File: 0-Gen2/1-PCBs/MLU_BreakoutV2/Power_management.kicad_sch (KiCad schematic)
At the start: 11 parts, among them J6 430450228, SW1 09.03201.02, U1 BA033CC0FP-E2

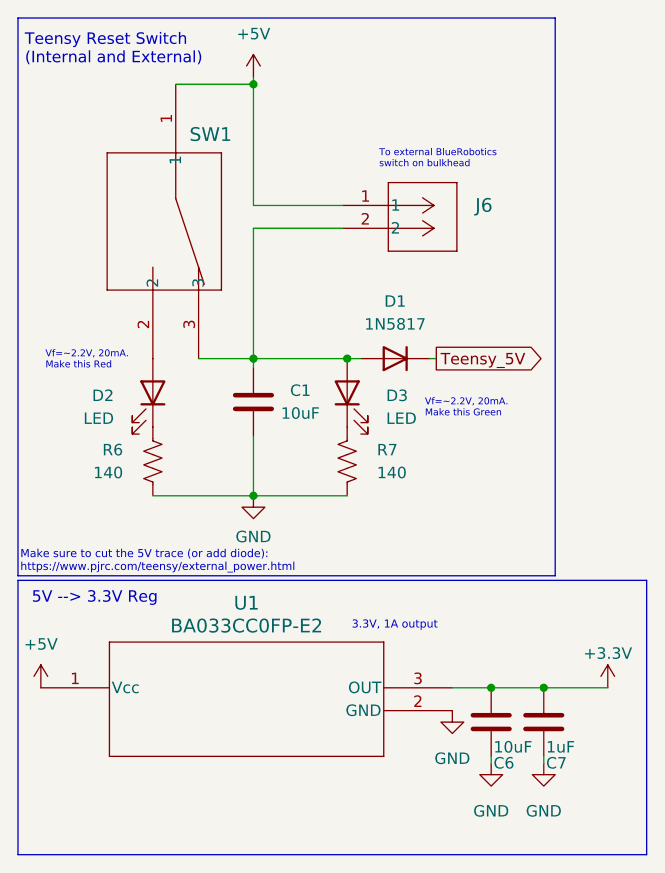
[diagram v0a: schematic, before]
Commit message: before restructure
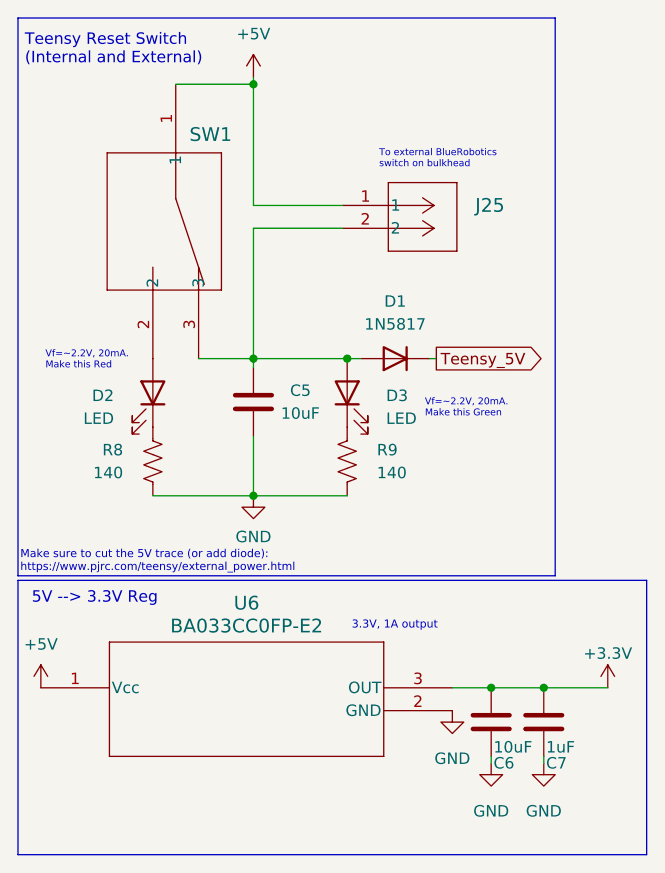
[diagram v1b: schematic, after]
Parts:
- renumbered C1 to C5, J6 to J25, R6 to R8, R7 to R9, U1 to U6
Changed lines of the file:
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@@
 		(dnp no)
 		(fields_autoplaced yes)
-		(property "Reference" "#PWR024"
+		(property "Reference" "#PWR0147"
 			(at 143.002 64.008 0)
 			(effects
@@
 			(project "MLU_BreakoutV2"
 				(path "/55121ba7-5d22-4fe3-93aa-7f76d75b410c/9e78e214-9eaa-4133-a14f-75961ce763bc"
-					(reference "#PWR024")
+					(reference "#PWR0147")
 					(unit 1)
 				)
@@
 		(dnp no)
 		(fields_autoplaced yes)
-		(property "Reference" "#PWR053"
+		(property "Reference" "#PWR0152"
 			(at 169.418 142.748 0)
 			(effects
@@
 			(project "MLU_BreakoutV2"
 				(path "/55121ba7-5d22-4fe3-93aa-7f76d75b410c/9e78e214-9eaa-4133-a14f-75961ce763bc"
-					(reference "#PWR053")
+					(reference "#PWR0152")
 					(unit 1)
 				)
@@
 		(dnp no)
 		(fields_autoplaced yes)
-		(property "Reference" "#PWR042"
+		(property "Reference" "#PWR0149"
 			(at 119.38 131.826 0)
 			(effects
@@
 			(project "MLU_BreakoutV2"
 				(path "/55121ba7-5d22-4fe3-93aa-7f76d75b410c/9e78e214-9eaa-4133-a14f-75961ce763bc"
-					(reference "#PWR042")
+					(reference "#PWR0149")
 					(unit 1)
 				)
@@
 		(dnp no)
 		(fields_autoplaced yes)
-		(property "Reference" "#PWR044"
+		(property "Reference" "#PWR0151"
 			(at 165.1 136.906 0)
 			(effects
@@
 			(project "MLU_BreakoutV2"
 				(path "/55121ba7-5d22-4fe3-93aa-7f76d75b410c/9e78e214-9eaa-4133-a14f-75961ce763bc"
-					(reference "#PWR044")
+					(reference "#PWR0151")
 					(unit 1)
 				)
@@
 		(dnp no)
 		(fields_autoplaced yes)
-		(property "Reference" "J6"
+		(property "Reference" "J25"
 			(at 167.64 74.4219 0)
 			(effects
@@
 			(project "MLU_BreakoutV2"
 				(path "/55121ba7-5d22-4fe3-93aa-7f76d75b410c/9e78e214-9eaa-4133-a14f-75961ce763bc"
-					(reference "J6")
+					(reference "J25")
 					(unit 1)
 				)
@@
 		(on_board yes)
 		(dnp no)
-		(property "Reference" "R7"
+		(property "Reference" "R9"
 			(at 156.718 101.5999 0)
 			(effects
@@
 			(project "MLU_BreakoutV2"
 				(path "/55121ba7-5d22-4fe3-93aa-7f76d75b410c/9e78e214-9eaa-4133-a14f-75961ce763bc"
-					(reference "R7")
+					(reference "R9")
 					(unit 1)
 				)
@@
 		(dnp no)
 		(fields_autoplaced yes)
-		(property "Reference" "U1"
+		(property "Reference" "U6"
 			(at 142.24 118.618 0)
 			(effects
@@
 			(project "MLU_BreakoutV2"
 				(path "/55121ba7-5d22-4fe3-93aa-7f76d75b410c/9e78e214-9eaa-4133-a14f-75961ce763bc"
-					(reference "U1")
+					(reference "U6")
 					(unit 1)
 				)
@@
 		(dnp no)
 		(fields_autoplaced yes)
-		(property "Reference" "#PWR054"
+		(property "Reference" "#PWR0153"
 			(at 175.26 142.748 0)
 			(effects
@@
 			(project "MLU_BreakoutV2"
 				(path "/55121ba7-5d22-4fe3-93aa-7f76d75b410c/9e78e214-9eaa-4133-a14f-75961ce763bc"
-					(reference "#PWR054")
+					(reference "#PWR0153")
 					(unit 1)
 				)
@@
 		(dnp no)
 		(fields_autoplaced yes)
-		(property "Reference" "#PWR037"
+		(property "Reference" "#PWR0148"
 			(at 143.002 113.03 0)
 			(effects
@@
 			(project "MLU_BreakoutV2"
 				(path "/55121ba7-5d22-4fe3-93aa-7f76d75b410c/9e78e214-9eaa-4133-a14f-75961ce763bc"
-					(reference "#PWR037")
+					(reference "#PWR0148")
 					(unit 1)
 				)
@@
 		(on_board yes)
 		(dnp no)
-		(property "Reference" "R6"
+		(property "Reference" "R8"
 			(at 128.524 101.5999 0)
 			(effects
@@
 			(project "MLU_BreakoutV2"
 				(path "/55121ba7-5d22-4fe3-93aa-7f76d75b410c/9e78e214-9eaa-4133-a14f-75961ce763bc"
-					(reference "R6")
+					(reference "R8")
 					(unit 1)
 				)
@@
 		(on_board yes)
 		(dnp no)
-		(property "Reference" "C1"
+		(property "Reference" "C5"
 			(at 147.066 94.9959 0)
 			(effects
@@
 			(project "MLU_BreakoutV2"
 				(path "/55121ba7-5d22-4fe3-93aa-7f76d75b410c/9e78e214-9eaa-4133-a14f-75961ce763bc"
-					(reference "C1")
+					(reference "C5")
 					(unit 1)
 				)
@@
 		(on_board yes)
 		(dnp no)
-		(property "Reference" "#PWR043"
+		(property "Reference" "#PWR0150"
 			(at 182.372 131.826 0)
 			(effects
@@
 			(project "MLU_BreakoutV2"
 				(path "/55121ba7-5d22-4fe3-93aa-7f76d75b410c/9e78e214-9eaa-4133-a14f-75961ce763bc"
-					(reference "#PWR043")
+					(reference "#PWR0150")
 					(unit 1)
 				)
